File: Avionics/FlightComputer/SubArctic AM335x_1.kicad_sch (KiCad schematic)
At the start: 1 part

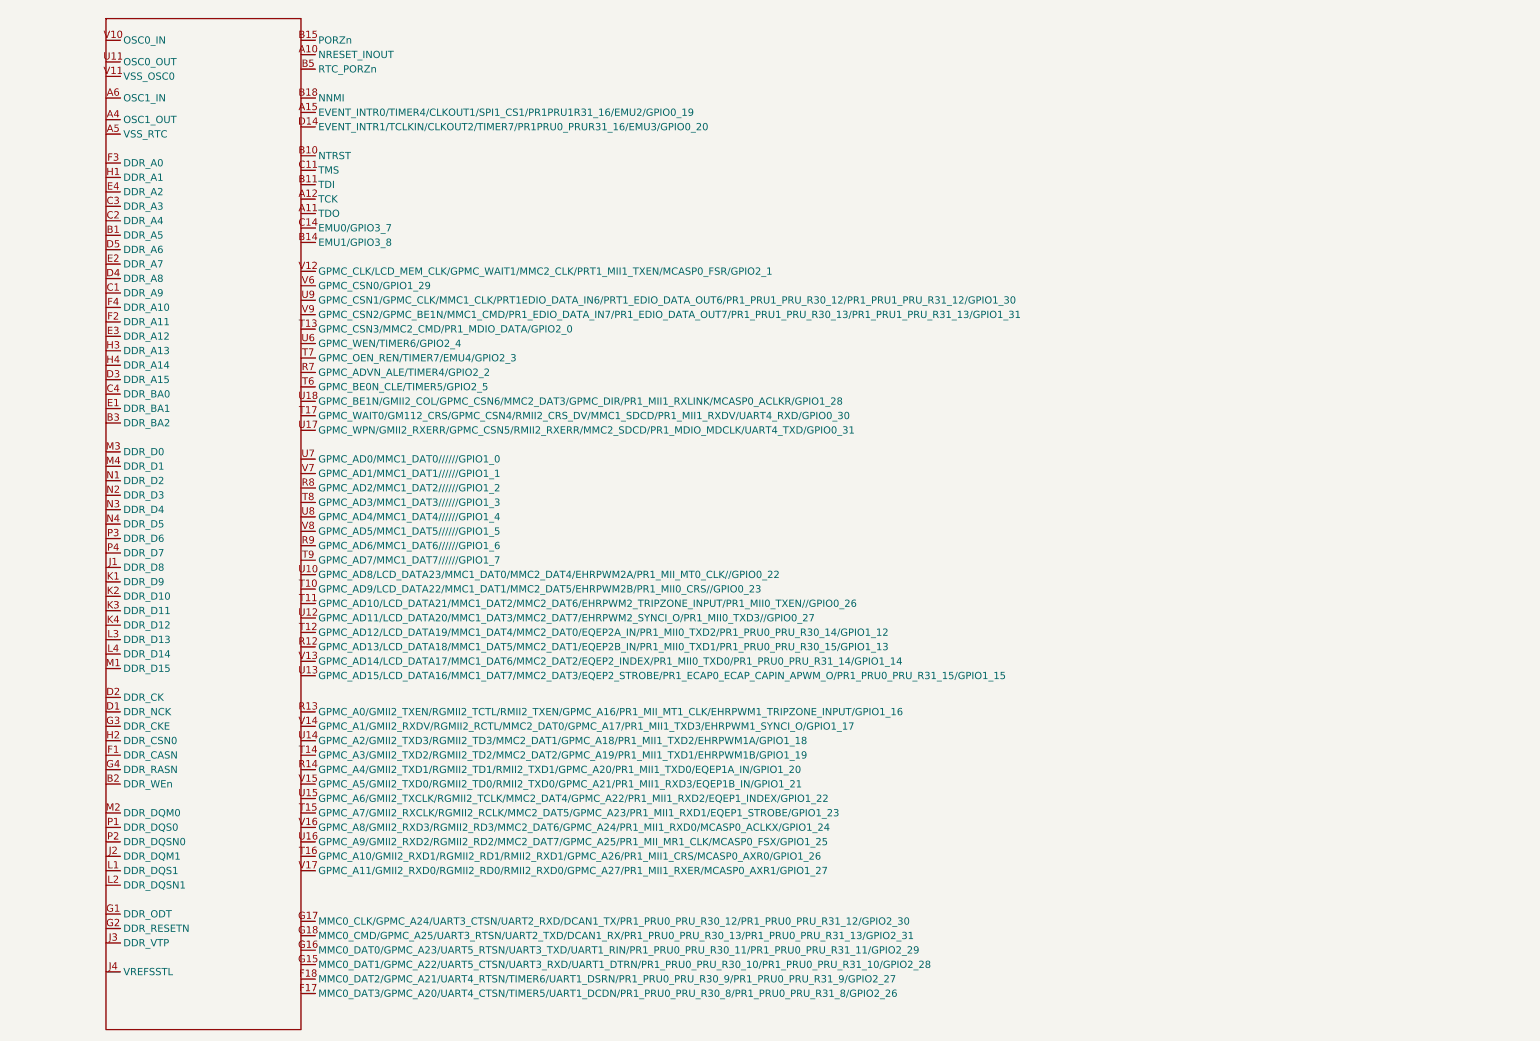
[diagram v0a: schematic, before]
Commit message: Ian Goldberg - Made substantial additions to the main chip of the flight computer. Wrapping up progress for the night.
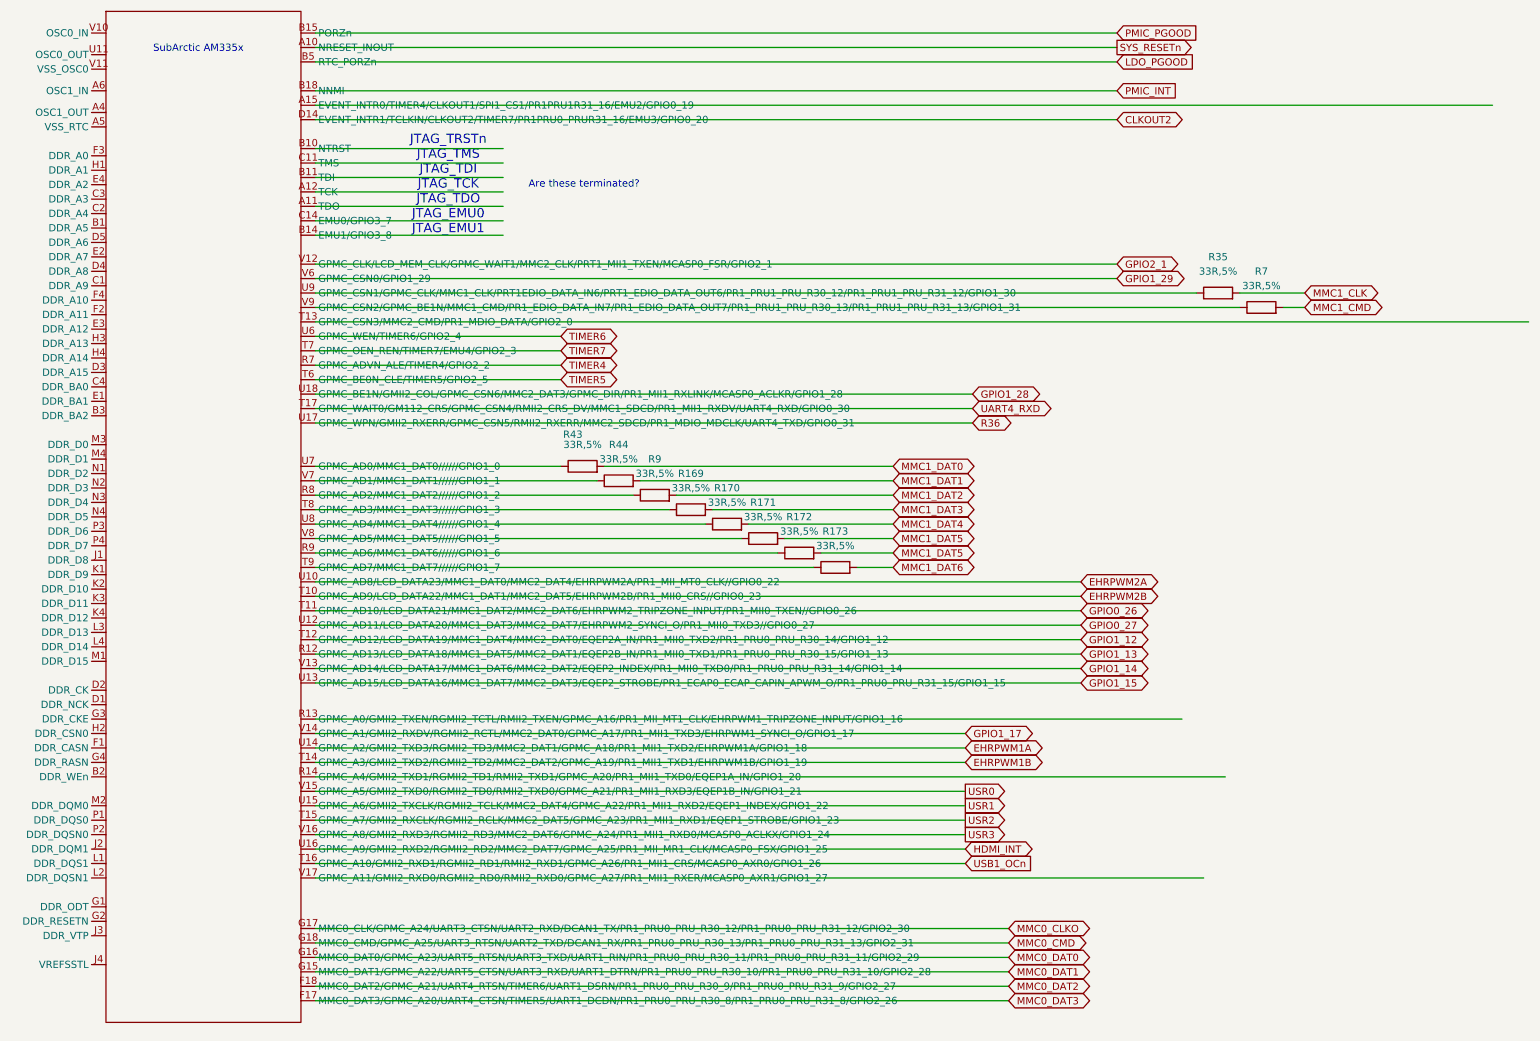
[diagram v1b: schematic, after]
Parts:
- added R169, R170, R171, R172, R173, R35, R43, R44, R7, R9: 33R,5%, symbol Device:R
- renumbered U2 to SubArcticAM335X
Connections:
- new net MMC1_CLK: R35.2
- new net MMC1_CMD: R7.2
- new net MMC1_DAT0: R43.2
- new net MMC1_DAT1: R44.2
- new net MMC1_DAT2: R9.2
- new net MMC1_DAT3: R169.2
- new net MMC1_DAT4: R170.2
- new net MMC1_DAT5: R171.2, R172.2
- new net MMC1_DAT6: R173.2
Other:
- note added: "Are these terminated?"
- note added: "JTAG_TRSTn JTAG_TMS JTAG_TDI JTAG_TCK JTAG_TDO JTAG_EMU0 JTAG_EMU1"
- note added: "SubArctic AM335x"
